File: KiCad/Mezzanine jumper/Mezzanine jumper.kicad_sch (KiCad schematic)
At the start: 2 parts, among them J1 Conn_02x50_Row_Letter_First, J2 Conn_02x50_Row_Letter_First

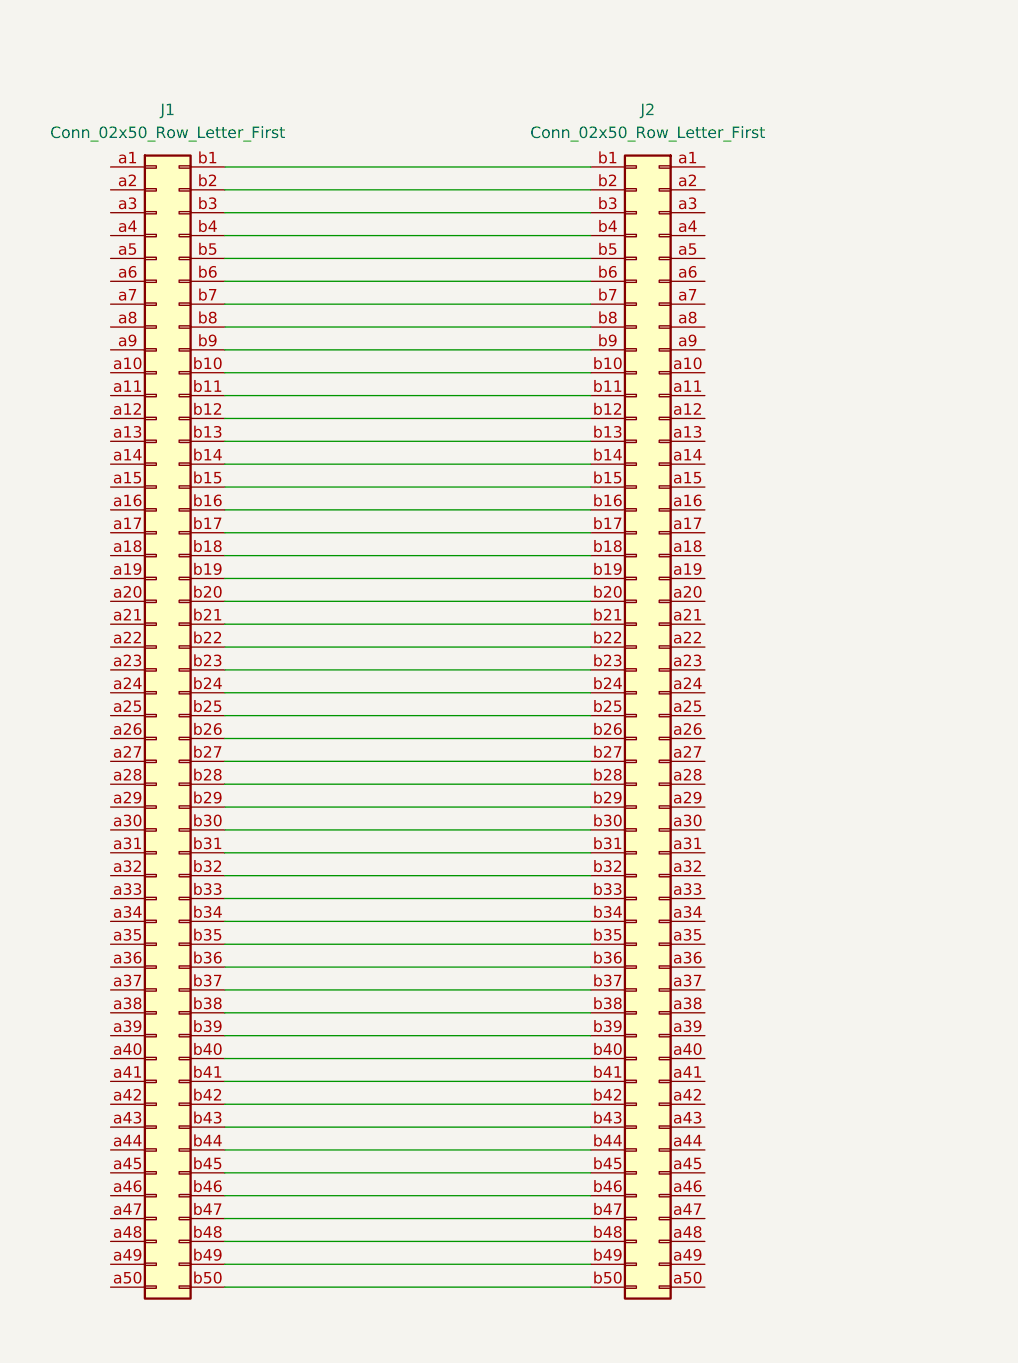
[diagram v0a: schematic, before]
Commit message: update boards
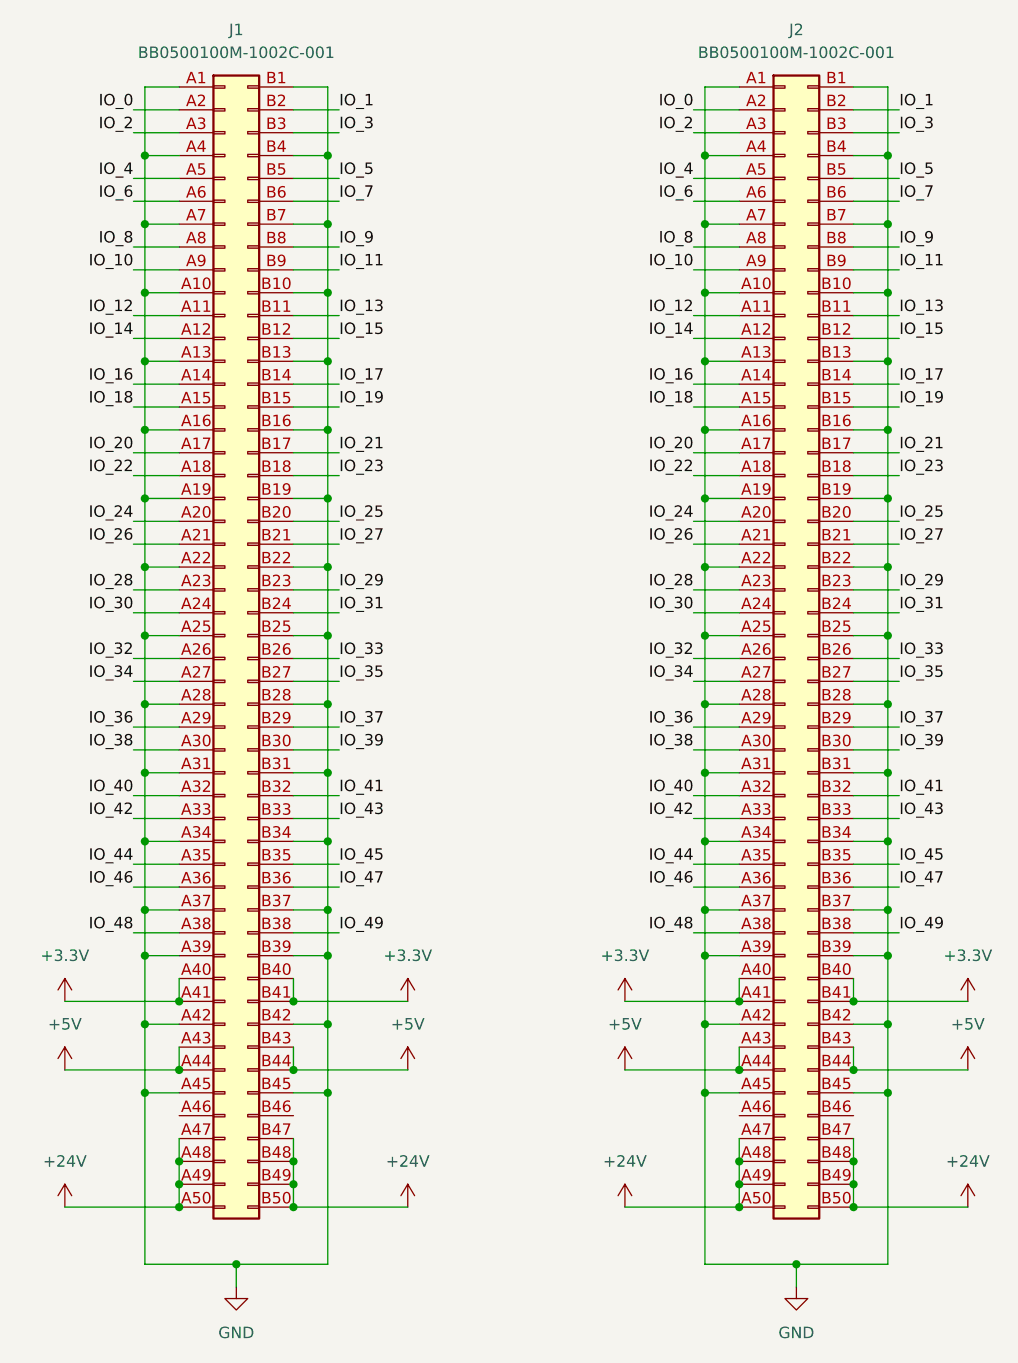
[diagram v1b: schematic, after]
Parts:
- removed J1, J2: Conn_02x50_Row_Letter_First, symbol Connector_Generic:Conn_02x50_Row_Letter_First
- added J1, J2: BB0500100M-1002C-001, footprints:BB0500100M-1002C-001, symbol symbols:Conn_02x50_Row_Letter_First
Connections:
- new net +24V: J1.A47 (Pin_A47), J1.A48 (Pin_A48), J1.A49 (Pin_A49), J1.A50 (Pin_A50), J1.B47 (Pin_B47), J1.B48 (Pin_B48), J1.B49 (Pin_B49), J1.B50 (Pin_B50), J2.A47 (Pin_A47), J2.A48 (Pin_A48), J2.A49 (Pin_A49), J2.A50 (Pin_A50), J2.B47 (Pin_B47), J2.B48 (Pin_B48), J2.B49 (Pin_B49), J2.B50 (Pin_B50)
- new net +3.3V: J1.A40 (Pin_A40), J1.A41 (Pin_A41), J1.B40 (Pin_B40), J1.B41 (Pin_B41), J2.A40 (Pin_A40), J2.A41 (Pin_A41), J2.B40 (Pin_B40), J2.B41 (Pin_B41)
- new net +5V: J1.A43 (Pin_A43), J1.A44 (Pin_A44), J1.B43 (Pin_B43), J1.B44 (Pin_B44), J2.A43 (Pin_A43), J2.A44 (Pin_A44), J2.B43 (Pin_B43), J2.B44 (Pin_B44)
- new net GND: J1.A1 (Pin_A1), J1.A10 (Pin_A10), J1.A13 (Pin_A13), J1.A16 (Pin_A16), J1.A19 (Pin_A19), J1.A22 (Pin_A22), J1.A25 (Pin_A25), J1.A28 (Pin_A28), J1.A31 (Pin_A31), J1.A34 (Pin_A34), J1.A37 (Pin_A37), J1.A39 (Pin_A39), J1.A4 (Pin_A4), J1.A42 (Pin_A42), J1.A45 (Pin_A45), J1.A7 (Pin_A7), J1.B1 (Pin_B1), J1.B10 (Pin_B10), J1.B13 (Pin_B13), J1.B16 (Pin_B16), J1.B19 (Pin_B19), J1.B22 (Pin_B22), J1.B25 (Pin_B25), J1.B28 (Pin_B28), J1.B31 (Pin_B31), J1.B34 (Pin_B34), J1.B37 (Pin_B37), J1.B39 (Pin_B39), J1.B4 (Pin_B4), J1.B42 (Pin_B42), J1.B45 (Pin_B45), J1.B7 (Pin_B7), J2.A1 (Pin_A1), J2.A10 (Pin_A10), J2.A13 (Pin_A13), J2.A16 (Pin_A16), J2.A19 (Pin_A19), J2.A22 (Pin_A22), J2.A25 (Pin_A25), J2.A28 (Pin_A28), J2.A31 (Pin_A31), J2.A34 (Pin_A34), J2.A37 (Pin_A37), J2.A39 (Pin_A39), J2.A4 (Pin_A4), J2.A42 (Pin_A42), J2.A45 (Pin_A45), J2.A7 (Pin_A7), J2.B1 (Pin_B1), J2.B10 (Pin_B10), J2.B13 (Pin_B13), J2.B16 (Pin_B16), J2.B19 (Pin_B19), J2.B22 (Pin_B22), J2.B25 (Pin_B25), J2.B28 (Pin_B28), J2.B31 (Pin_B31), J2.B34 (Pin_B34), J2.B37 (Pin_B37), J2.B39 (Pin_B39), J2.B4 (Pin_B4), J2.B42 (Pin_B42), J2.B45 (Pin_B45), J2.B7 (Pin_B7)
- new net IO_0: J1.A2 (Pin_A2), J2.A2 (Pin_A2)
- new net IO_1: J1.B2 (Pin_B2), J2.B2 (Pin_B2)
- new net IO_10: J1.A9 (Pin_A9), J2.A9 (Pin_A9)
- new net IO_11: J1.B9 (Pin_B9), J2.B9 (Pin_B9)
- new net IO_12: J1.A11 (Pin_A11), J2.A11 (Pin_A11)
- new net IO_13: J1.B11 (Pin_B11), J2.B11 (Pin_B11)
- new net IO_14: J1.A12 (Pin_A12), J2.A12 (Pin_A12)
- new net IO_15: J1.B12 (Pin_B12), J2.B12 (Pin_B12)
- new net IO_16: J1.A14 (Pin_A14), J2.A14 (Pin_A14)
- new net IO_17: J1.B14 (Pin_B14), J2.B14 (Pin_B14)
- new net IO_18: J1.A15 (Pin_A15), J2.A15 (Pin_A15)
- new net IO_19: J1.B15 (Pin_B15), J2.B15 (Pin_B15)
- new net IO_2: J1.A3 (Pin_A3), J2.A3 (Pin_A3)
- new net IO_20: J1.A17 (Pin_A17), J2.A17 (Pin_A17)
- new net IO_21: J1.B17 (Pin_B17), J2.B17 (Pin_B17)
- new net IO_22: J1.A18 (Pin_A18), J2.A18 (Pin_A18)
- new net IO_23: J1.B18 (Pin_B18), J2.B18 (Pin_B18)
- new net IO_24: J1.A20 (Pin_A20), J2.A20 (Pin_A20)
- new net IO_25: J1.B20 (Pin_B20), J2.B20 (Pin_B20)
- new net IO_26: J1.A21 (Pin_A21), J2.A21 (Pin_A21)
- new net IO_27: J1.B21 (Pin_B21), J2.B21 (Pin_B21)
- new net IO_28: J1.A23 (Pin_A23), J2.A23 (Pin_A23)
- new net IO_29: J1.B23 (Pin_B23), J2.B23 (Pin_B23)
- new net IO_3: J1.B3 (Pin_B3), J2.B3 (Pin_B3)
- new net IO_30: J1.A24 (Pin_A24), J2.A24 (Pin_A24)
- new net IO_31: J1.B24 (Pin_B24), J2.B24 (Pin_B24)
- new net IO_32: J1.A26 (Pin_A26), J2.A26 (Pin_A26)
- new net IO_33: J1.B26 (Pin_B26), J2.B26 (Pin_B26)
- new net IO_34: J1.A27 (Pin_A27), J2.A27 (Pin_A27)
- new net IO_35: J1.B27 (Pin_B27), J2.B27 (Pin_B27)
- new net IO_36: J1.A29 (Pin_A29), J2.A29 (Pin_A29)
- new net IO_37: J1.B29 (Pin_B29), J2.B29 (Pin_B29)
- new net IO_38: J1.A30 (Pin_A30), J2.A30 (Pin_A30)
- new net IO_39: J1.B30 (Pin_B30), J2.B30 (Pin_B30)
- new net IO_4: J1.A5 (Pin_A5), J2.A5 (Pin_A5)
- new net IO_40: J1.A32 (Pin_A32), J2.A32 (Pin_A32)
- new net IO_41: J1.B32 (Pin_B32), J2.B32 (Pin_B32)
- new net IO_42: J1.A33 (Pin_A33), J2.A33 (Pin_A33)
- new net IO_43: J1.B33 (Pin_B33), J2.B33 (Pin_B33)
- new net IO_44: J1.A35 (Pin_A35), J2.A35 (Pin_A35)
- new net IO_45: J1.B35 (Pin_B35), J2.B35 (Pin_B35)
- new net IO_46: J1.A36 (Pin_A36), J2.A36 (Pin_A36)
- new net IO_47: J1.B36 (Pin_B36), J2.B36 (Pin_B36)
- new net IO_48: J1.A38 (Pin_A38), J2.A38 (Pin_A38)
- new net IO_49: J1.B38 (Pin_B38), J2.B38 (Pin_B38)
- new net IO_5: J1.B5 (Pin_B5), J2.B5 (Pin_B5)
- new net IO_6: J1.A6 (Pin_A6), J2.A6 (Pin_A6)
- new net IO_7: J1.B6 (Pin_B6), J2.B6 (Pin_B6)
- new net IO_8: J1.A8 (Pin_A8), J2.A8 (Pin_A8)
- new net IO_9: J1.B8 (Pin_B8), J2.B8 (Pin_B8)
